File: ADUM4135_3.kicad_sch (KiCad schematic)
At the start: 36 parts, among them Q10 MJD45H11T4G, Q11 MJD44H11T4G, Q12 MJD45H11T4G, Q9 MJD44H11T4G

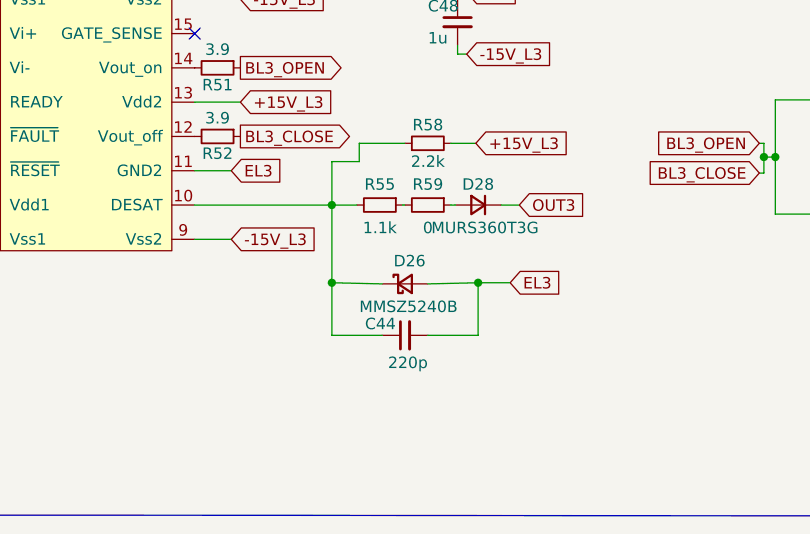
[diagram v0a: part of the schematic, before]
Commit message: Нашёл ошибки
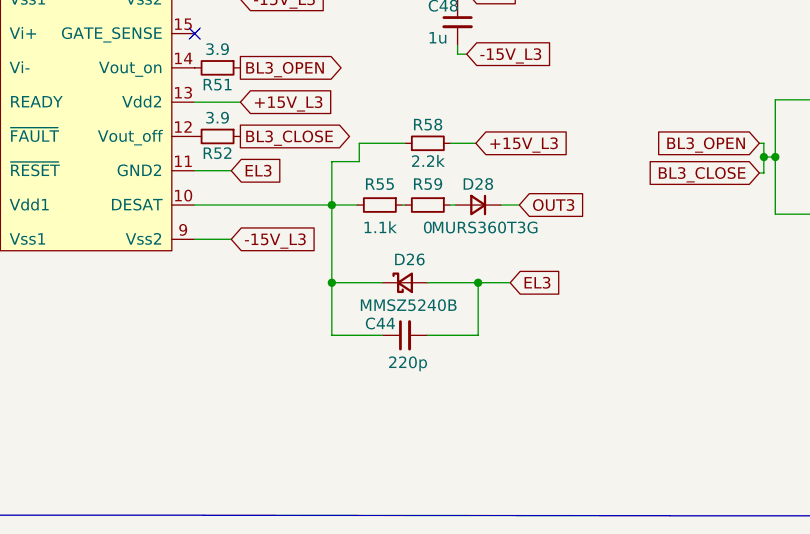
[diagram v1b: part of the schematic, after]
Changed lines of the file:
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@@
     (stroke (width 0) (type default) (color 0 0 0 0))
   )
-  (wire (pts (xy 115.57 155.575) (xy 109.982 155.448))
+  (wire (pts (xy 115.57 155.448) (xy 109.982 155.448))
     (stroke (width 0) (type default) (color 0 0 0 0))
   )
@@
     (stroke (width 0) (type default) (color 0 0 0 0))
   )
-  (wire (pts (xy 120.65 155.575) (xy 126.238 155.448))
+  (wire (pts (xy 120.65 155.448) (xy 126.238 155.448))
     (stroke (width 0) (type default) (color 0 0 0 0))
   )
@@
     (pin "1")
   )
-  (symbol (lib_id "Device:D_Schottky_Small") (at 118.11 155.575 0) (unit 1)
-    (in_bom yes) (on_board yes)
-    (property "Reference" "D26" (id 0) (at 116.84 153.035 0)
-      (effects (font (size 1.27 1.27)) (justify left))
-    )
-    (property "Value" "MMSZ5240B" (id 1) (at 113.03 158.115 0)
-      (effects (font (size 1.27 1.27)) (justify left))
-    )
-    (property "Footprint" "Diode_SMD:D_SOD-123" (id 2) (at 118.11 155.575 90)
-      (effects (font (size 1.27 1.27)) hide)
-    )
-    (property "Datasheet" "~" (id 3) (at 118.11 155.575 90)
-      (effects (font (size 1.27 1.27)) hide)
-    )
+  (symbol (lib_id "Device:D_Schottky_Small") (at 118.11 155.448 0) (unit 1)
+    (in_bom yes) (on_board yes)
+    (property "Reference" "D26" (id 0) (at 116.84 152.908 0)
+      (effects (font (size 1.27 1.27)) (justify left))
+    )
+    (property "Value" "MMSZ5240B" (id 1) (at 113.03 157.988 0)
+      (effects (font (size 1.27 1.27)) (justify left))
+    )
+    (property "Footprint" "Diode_SMD:D_SOD-123" (id 2) (at 118.11 155.448 90)
+      (effects (font (size 1.27 1.27)) hide)
+    )
+    (property "Datasheet" "~" (id 3) (at 118.11 155.448 90)
+      (effects (font (size 1.27 1.27)) hide)
+    )
